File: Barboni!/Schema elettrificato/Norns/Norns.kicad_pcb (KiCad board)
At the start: 2 copper layers, 65 x 56.5 mm, 27 parts, among them J1 Display, J2 Raspoberro, J3 Power Supply, J4 Encoders, J5 MIDI, J6 LED, Q1 S8550, Q2 2N7000, Q3 2N7000, U1 7404, U2 6N138

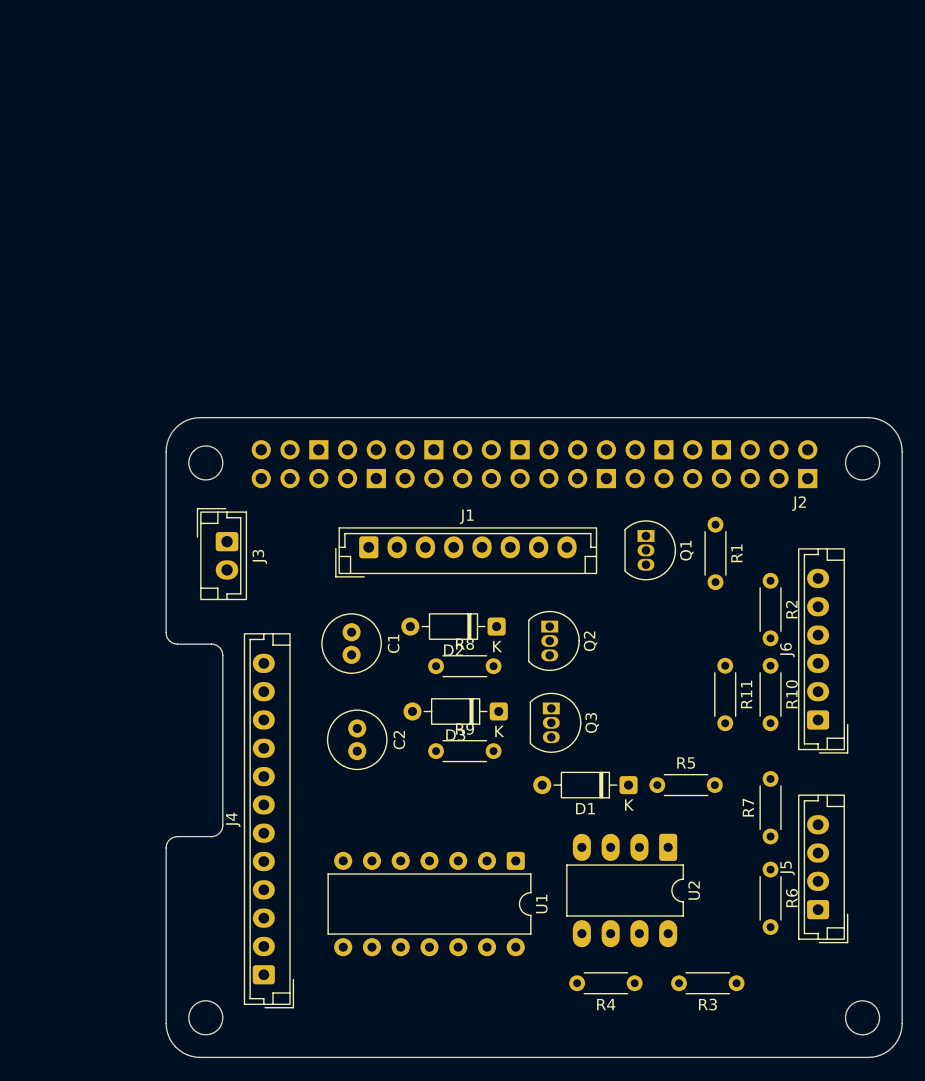
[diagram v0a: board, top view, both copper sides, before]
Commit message: ola
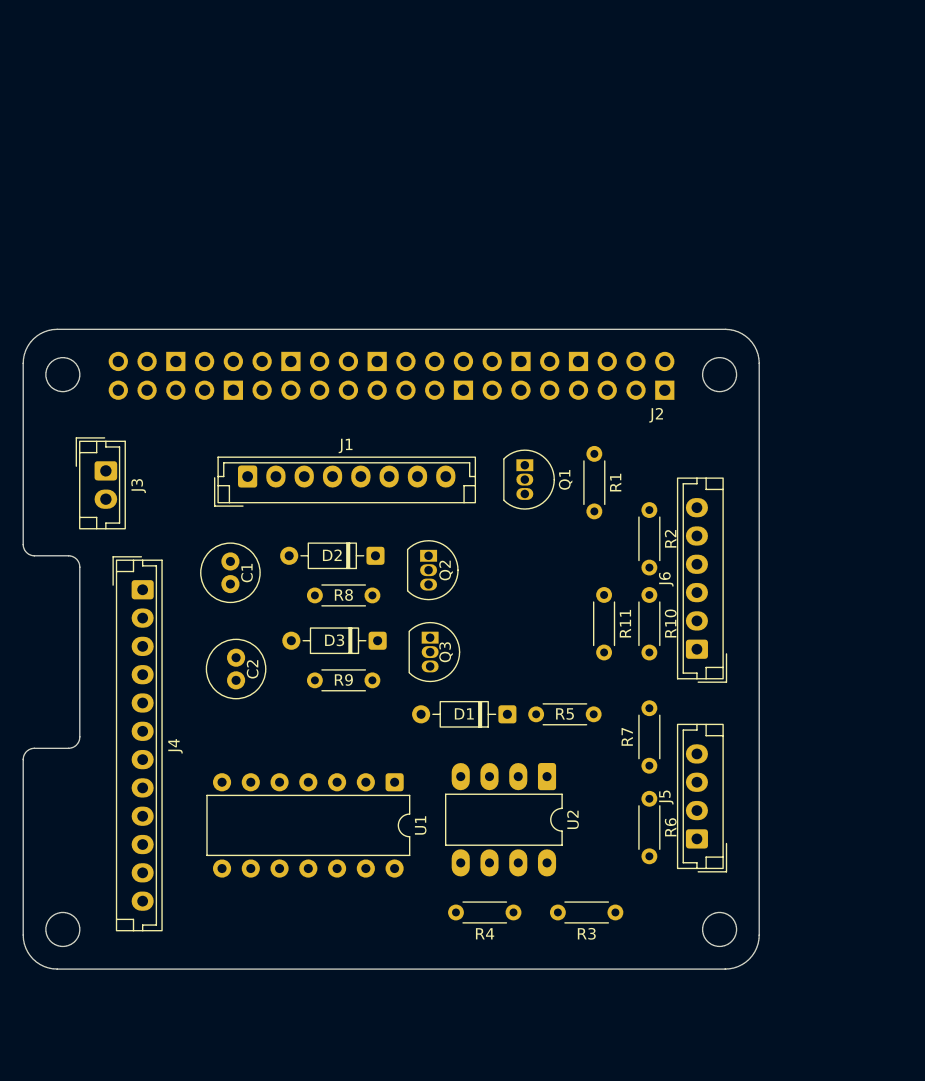
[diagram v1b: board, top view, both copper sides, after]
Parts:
- moved J4 35.6 mm to (75.5, 60.2), turned to -90 degrees
- moved J2 14.8 mm to (97.5, 41.2)
- moved U1 12.8 mm to (97.8, 77.2)
- moved C1 12.4 mm to (83.3, 57.8)
- moved C2 12.4 mm to (83.8, 66.2)
- moved D2 12.4 mm to (96.1, 57.2)
- moved D3 12.4 mm to (96.3, 64.8)
- moved J1 12.4 mm to (84.8, 50.2)
- moved J3 12.4 mm to (72.3, 49.8)
- moved Q1 12.4 mm to (109.3, 49.2)
- moved Q2 12.4 mm to (100.8, 57.2)
- moved Q3 12.4 mm to (100.9, 64.5)
- moved R1 12.4 mm to (115.4, 48.2)
- moved R2 12.4 mm to (120.3, 53.2)
- moved R3 12.4 mm to (117.3, 88.8)
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
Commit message: committamento
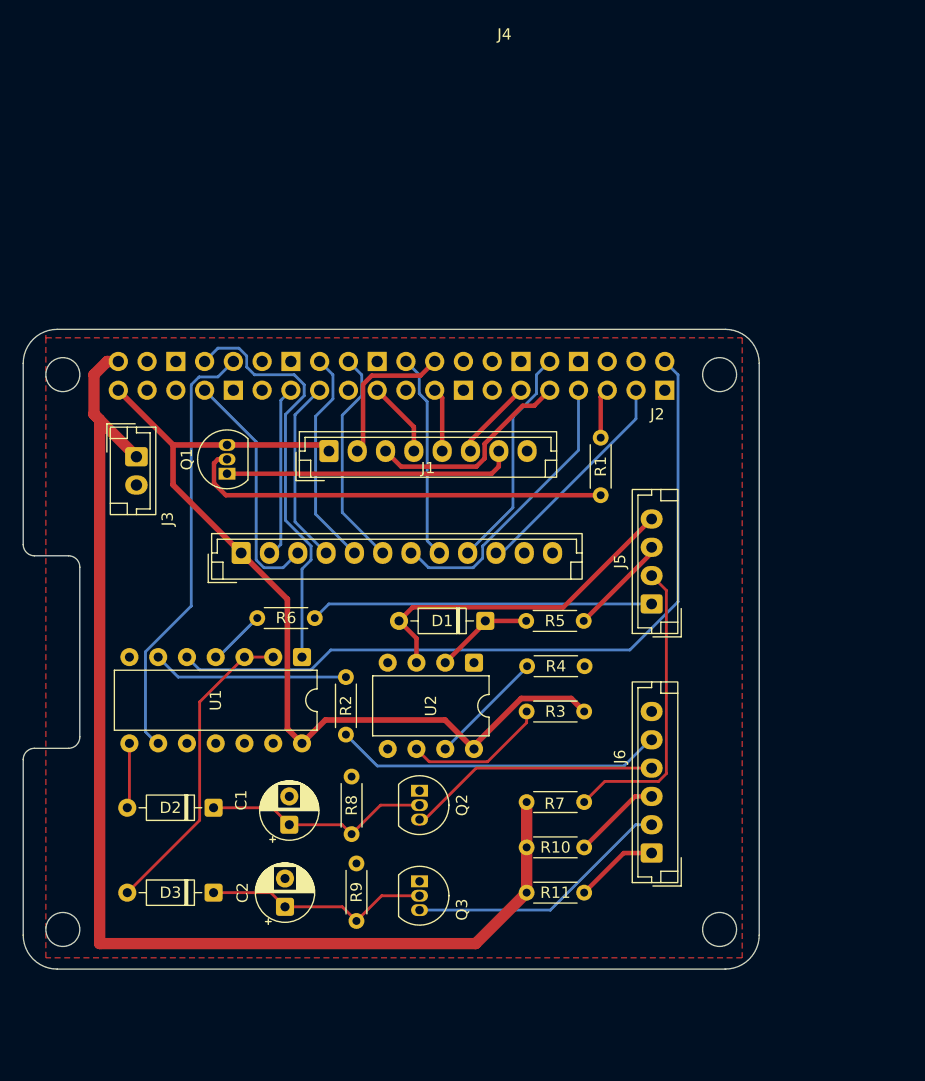
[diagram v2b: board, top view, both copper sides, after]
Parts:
- C1, C2: footprint Capacitor_THT:C_Radial_D5.0mm_H11.0mm_P2.00mm -> Capacitor_THT:CP_Radial_D5.0mm_P2.50mm
- U2: footprint Package_DIP:DIP-8_W7.62mm_LongPads -> Package_DIP:DIP-8_W7.62mm
- moved R6 38.1 mm to (85.7, 62.8), turned to 0 degrees
- moved R2 33.3 mm to (93.5, 73.0), turned to 90 degrees
- moved D3 26.6 mm to (81.8, 87.0)
- moved D2 26.4 mm to (81.8, 79.5)
- moved R11 26.3 mm to (114.5, 87.0), turned to 180 degrees
- moved Q1 26.3 mm to (83.0, 50.0), turned to 90 degrees
- moved C1 23.8 mm to (88.5, 81.0), turned to 90 degrees
- moved R10 23.0 mm to (114.5, 83.0), turned to 180 degrees
- moved C2 22.4 mm to (88.1, 88.2), turned to 90 degrees
- moved R4 21.8 mm to (109.5, 67.0), turned to 0 degrees
- moved Q3 21.5 mm to (100.0, 86.0)
- moved J5 21.1 mm to (120.5, 61.5)
- moved Q2 20.8 mm to (100.0, 78.0)
- moved J6 18.4 mm to (120.5, 83.5)
- moved R3 18.0 mm to (114.5, 71.0)
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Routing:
- net +5V: track 0.00 -> 106.0 mm
- net +3.3V: track 0.00 -> 81.2 mm
- net Net-(J2-BCM21_SCLK_PCM_DO): track 0.00 -> 68.0 mm
- net Net-(J2-BCM15_RXD): track 0.00 -> 51.2 mm
- net Net-(Q1-B): track 0.00 -> 37.7 mm
- net Net-(J2-BCM14_TXD): track 0.00 -> 37.2 mm
- net Net-(D1-A): track 0.00 -> 30.4 mm
- net Net-(J5-Pin_1): track 0.00 -> 30.3 mm
- net Net-(J6-Pin_5): track 0.00 -> 29.1 mm
- net Net-(D3-A): track 0.00 -> 27.6 mm
- net Net-(J5-Pin_2): track 0.00 -> 26.3 mm
- net Net-(J2-BCM13_PWM1): track 0.00 -> 25.9 mm
- net /LED_BL: track 0.00 -> 25.6 mm
- net Net-(J6-Pin_2): track 0.00 -> 23.6 mm
- net Net-(J6-Pin_4): track 0.00 -> 23.0 mm
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- added copper zone on F.Cu, net GND
